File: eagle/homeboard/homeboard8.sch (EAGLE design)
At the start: 77 parts, among them IC1 XCF02S, IC2 25LC080SN, IC3 ATMEGA32U2-TQFP, Q5 BC848SMD, Q6 BC848SMD, Q7 BC848SMD, Q8 BC848SMD, T1 BSS138, T2 BC848, T3 BSS138, U1 XC3S400TQ144, X1 1503_04, X2 SCART-F

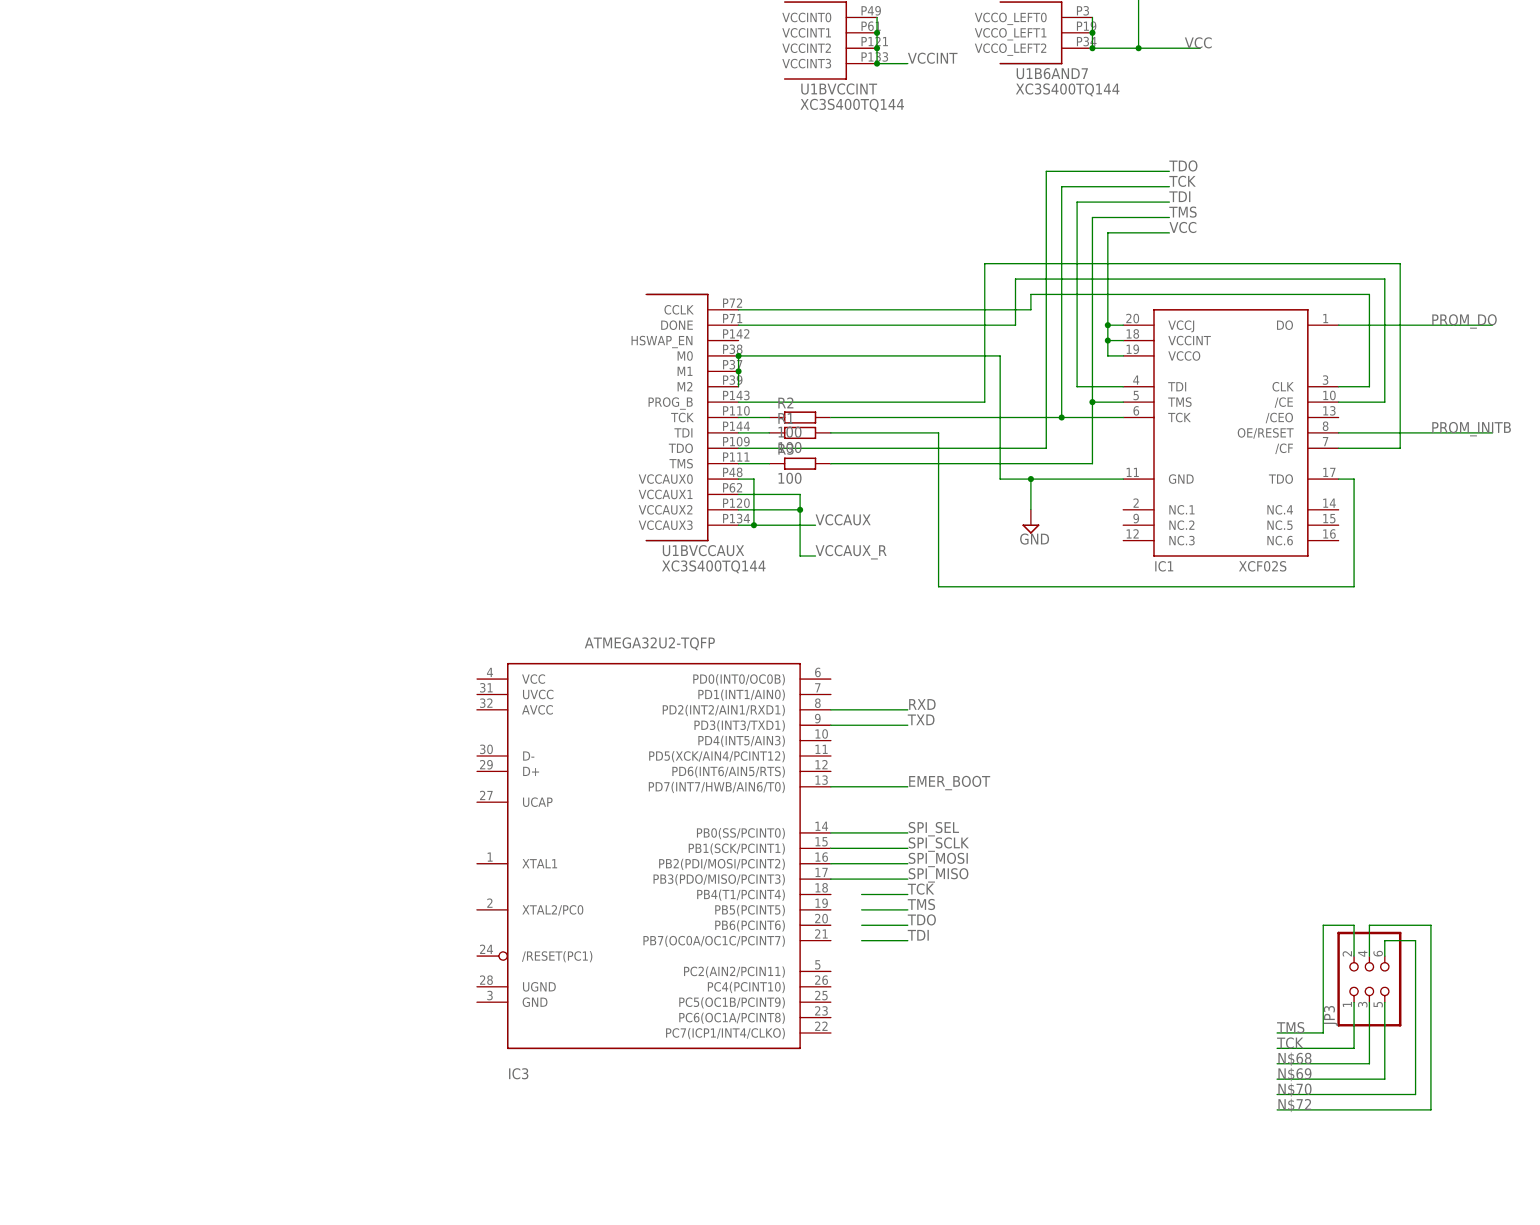
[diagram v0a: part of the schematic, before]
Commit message: rework
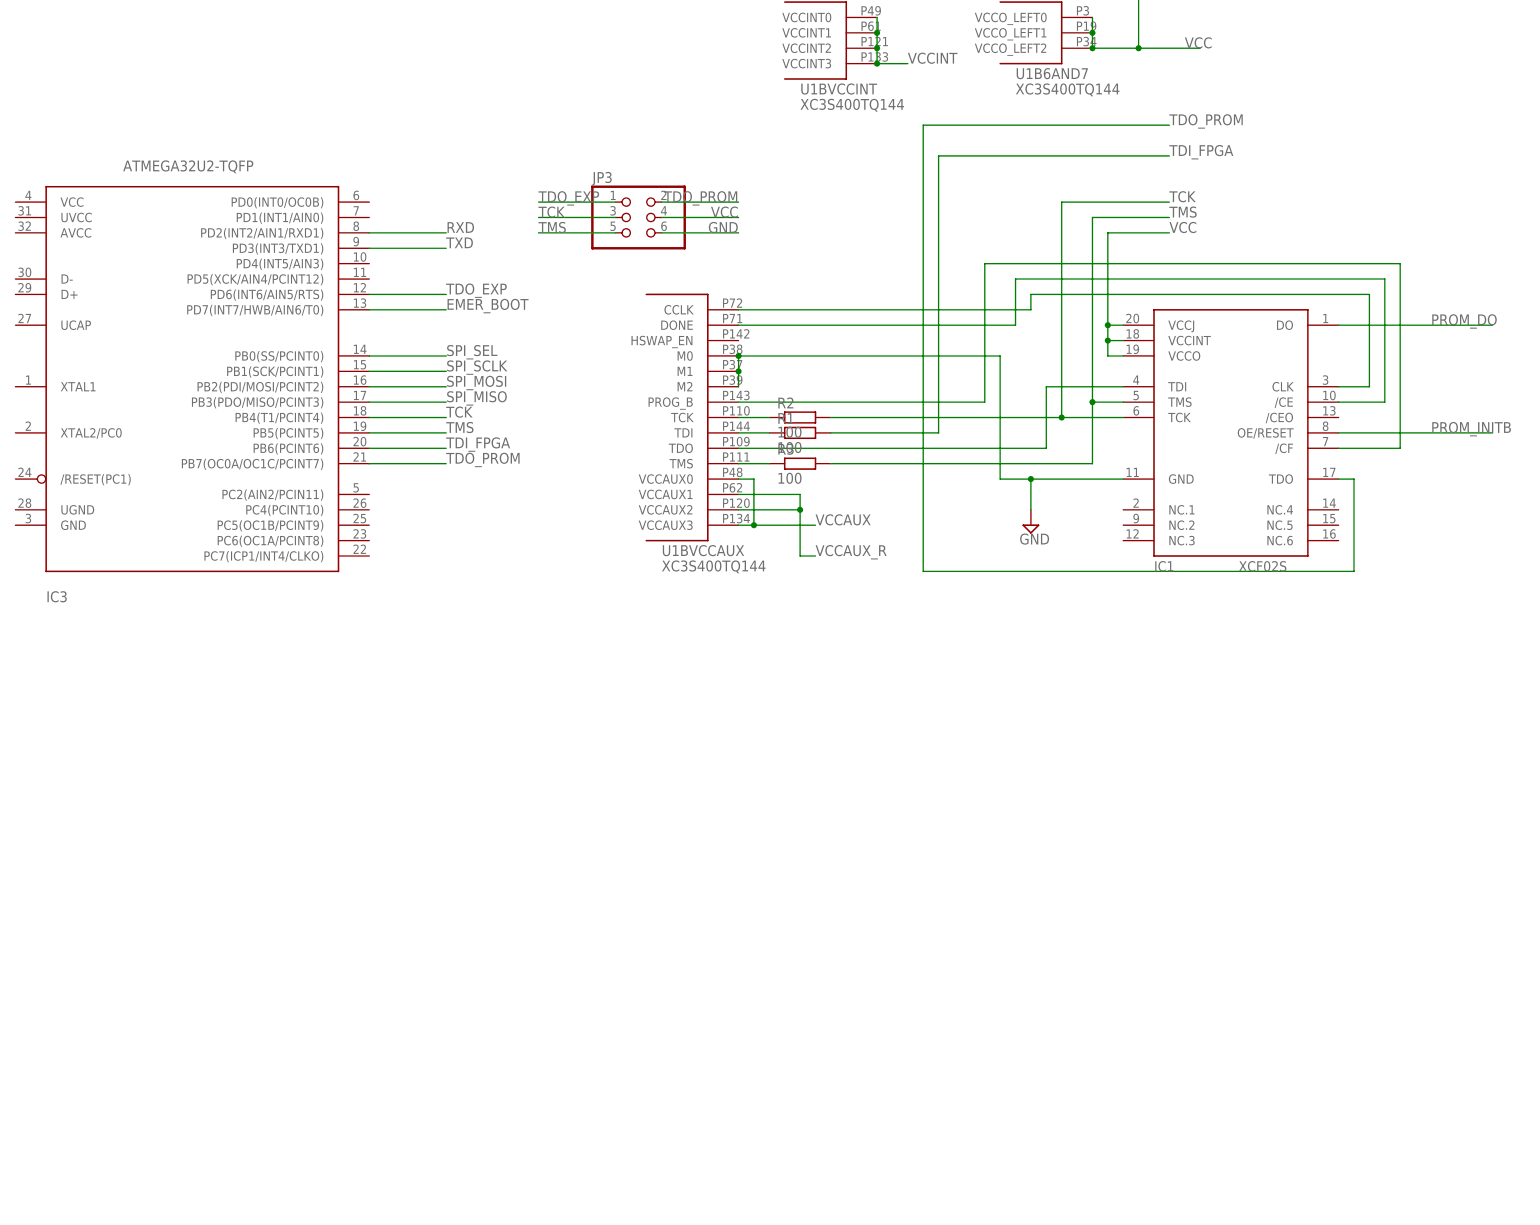
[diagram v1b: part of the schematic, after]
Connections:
- removed net N$36: IC1.TDO, R1.2
- removed net N$68: JP3.3
- removed net N$69: JP3.5
- removed net N$70: JP3.6
- removed net N$72: JP3.4
- removed net TDI: IC1.TDI
- removed net TDO: U1BVCCAUX.TDO
- new net SPI_MISO: IC3.PB3(PDO/MISO/PCINT3)
- new net SPI_MOSI: IC3.PB2(PDI/MOSI/PCINT2)
- new net SPI_SCLK: IC3.PB1(SCK/PCINT1)
- new net SPI_SEL: IC3.PB0(SS/PCINT0)
- new net TDI_FPGA: IC3.PB6(PCINT6), R1.2
- new net TDO_EXP: IC3.PD6(INT6/AIN5/RTS), JP3.1
- new net TDO_FPGA: IC1.TDI, U1BVCCAUX.TDO
- new net TDO_PROM: IC1.TDO, IC3.PB7(OC0A/OC1C/PCINT7), JP3.2
- net GND: now also JP3.6
- net TCK: now also IC3.PB4(T1/PCINT4), JP3.3; no longer JP3.1
- net TMS: now also IC3.PB5(PCINT5), JP3.5; no longer JP3.2
- net VCC: now also JP3.4
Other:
- moved on the sheet: IC3, JP3
